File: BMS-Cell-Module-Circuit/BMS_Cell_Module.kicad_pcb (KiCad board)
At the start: 2 copper layers, 45.7 x 65.8 mm, 35 parts, among them J1 Conn_01x02_Female, J2 Conn_01x04_Female, J3 Conn_01x04_Female, M1 SI2312BDS-T1-E3, U2 ADUM1250ARZ, U3 ATTINY85V-10SU 8S2 EIAJ SOIC

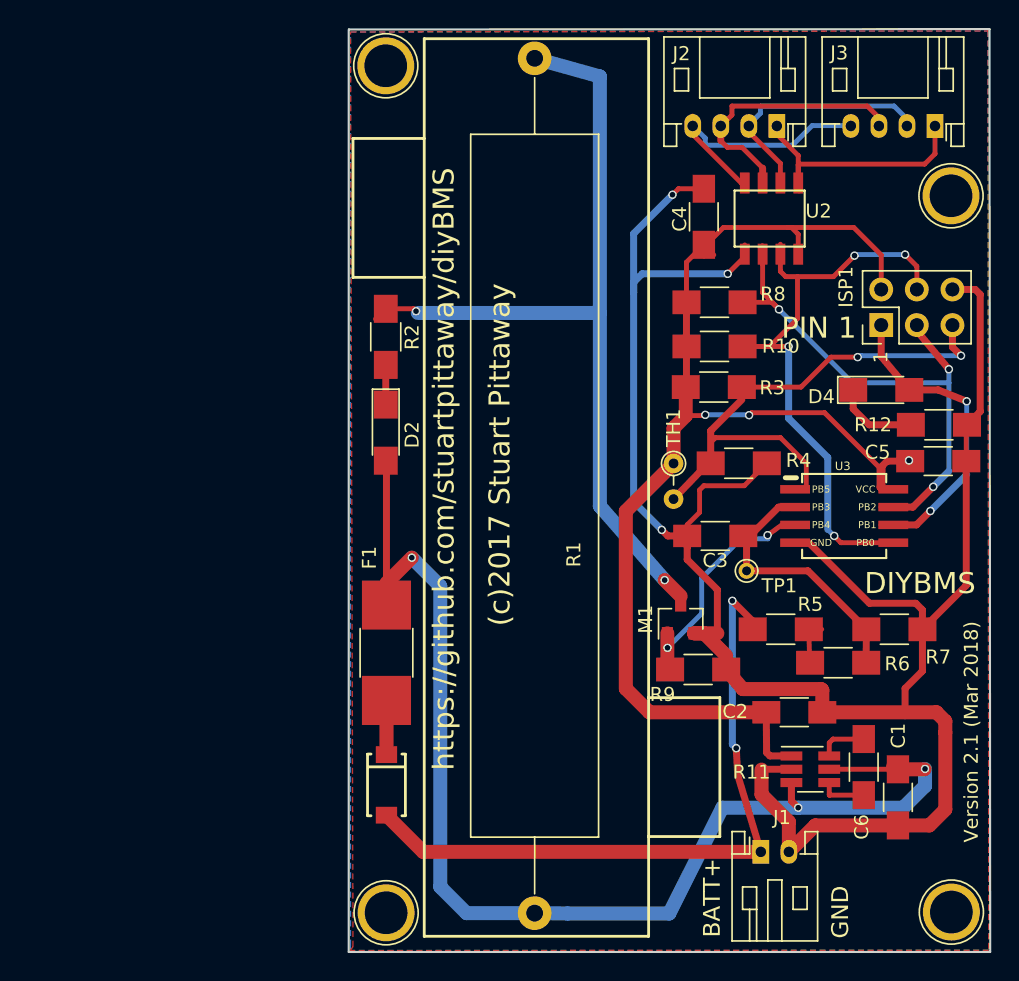
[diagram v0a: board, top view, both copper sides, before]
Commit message: First check in
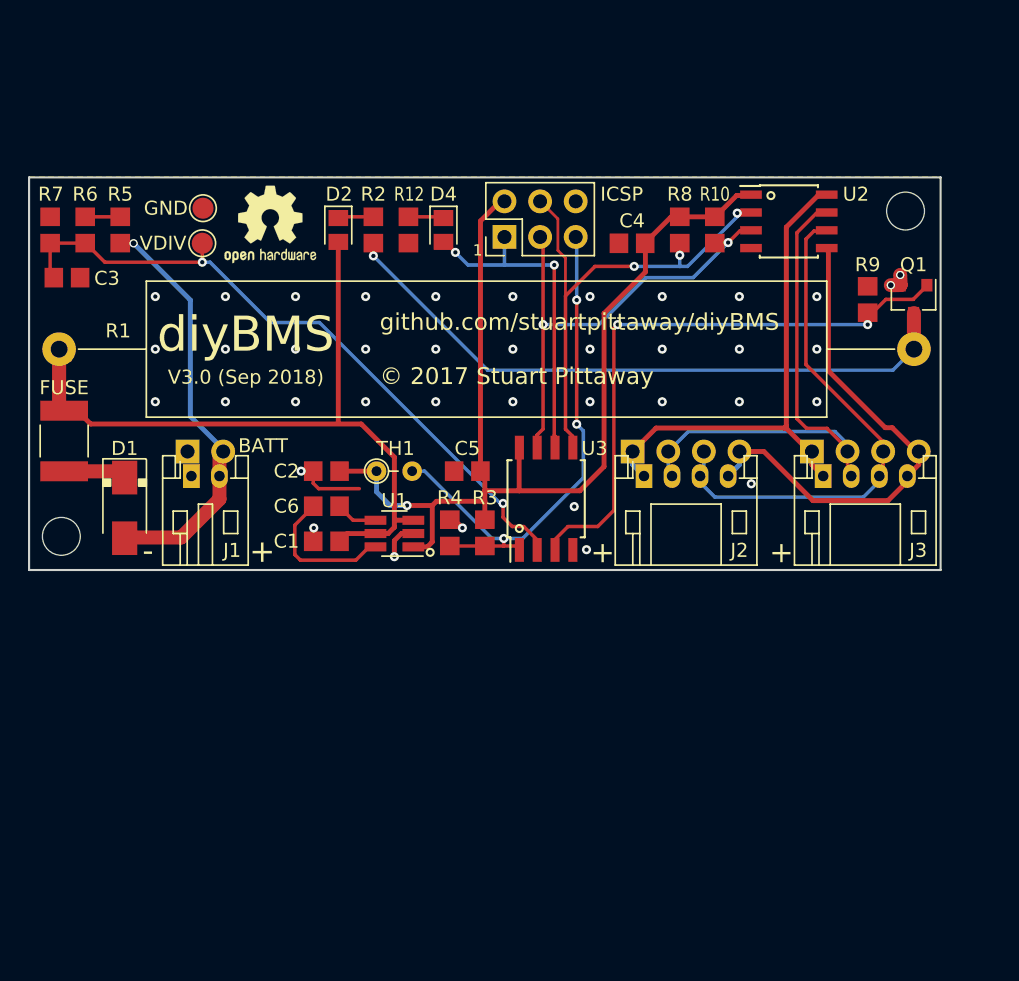
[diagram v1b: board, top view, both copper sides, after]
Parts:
- removed the J3 at (173.1, 67.3)
- removed M1: SI2312BDS-T1-E3, TO_SOT_Packages_SMD:SOT-23
- removed R11: REG710NA-3.3, TO_SOT_Packages_SMD:SOT-23-6_Handsoldering
- removed the REF** at (174.3, 123.4)
- removed the REF** at (134.0, 123.4)
- removed the REF** at (133.9, 63.0)
- added J2: Conn_01x04_Female, Connectors_JST:JST_PH_S4B-PH-K_04x2.00mm_Angled, F.Cu at (152.3, 92.3)
- added Q1: SI2312BDS-T1-E3, Package_TO_SOT_SMD:SOT-23, F.Cu at (171.6, 79.7)
- added REF**: PinHeader_1x04_P2.54mm_NoSilk, ATTINY:PinHeader_1x04_P2.54mm_NoSilk, F.Cu at (164.3, 90.5)
- added REF**: 2.7mm M2.5, MountingHole:MountingHole_2.7mm_M2.5, F.Cu at (110.8, 96.6)
- added REF**: OSHW-Logo2_7.3x6mm_SilkScreen, Symbol:OSHW-Logo2_7.3x6mm_SilkScreen, F.Cu at (125.7, 74.3)
- added REF**: PinHeader_1x04_P2.54mm_NoSilk, ATTINY:PinHeader_1x04_P2.54mm_NoSilk, F.Cu at (151.5, 90.5)
- added REF**: PinHeader_1x02_P2.54mm_NoSilk, ATTINY:PinHeader_1x02_P2.54mm_NoSilk, F.Cu at (119.8, 90.5)
- added TP2: TPGND, TestPoint:TestPoint_Pad_D1.5mm, F.Cu at (120.9, 73.2)
- added U1: REG710NA-3.3, TO_SOT_Packages_SMD:SOT-23-6_Handsoldering, F.Cu at (134.6, 96.4)
- C1, C2: value 2.2uF Ceramic X7R -> 2.2uF; footprint Capacitors_SMD:C_1206_HandSoldering -> Capacitor_SMD:C_0805_2012Metric_Pad1.33x1.40mm_HandSolder
- C3, C4, C5: footprint Capacitors_SMD:C_1206_HandSoldering -> Capacitor_SMD:C_0805_2012Metric_Pad1.33x1.40mm_HandSolder
- C6: value 0.22uF Ceramic X7R -> 0.22uF; footprint Capacitors_SMD:C_1206_HandSoldering -> Capacitor_SMD:C_0805_2012Metric_Pad1.33x1.40mm_HandSolder
- D1: value SE30AFG-M3/6A -> SS34 Schottky 40V/3A
- D2, D4: footprint LEDs:LED_1206_HandSoldering -> LED_SMD:LED_0805_2012Metric_Pad1.15x1.40mm_HandSolder
- F1: value MC36228 1.5A 8V -> FUSE; footprint Resistors_SMD:R_1812_HandSoldering -> Resistor_SMD:R_1812_4532Metric_Pad1.42x3.40mm_HandSolder
- R1: value HS50 3R3 J 50W Axial Wire Wound -> 2R/10W; footprint Resistors_THT:R_Axial_Power_L50.0mm_W9.0mm_P60.96mm -> ATTINY:R_Axial_Power_L48.0mm_W9.5mm_P60.96mm
- R10, R12, R4, R5, R6, R7, R8, R9: footprint Resistors_SMD:R_1206_HandSoldering -> Resistor_SMD:R_0805_2012Metric_Pad1.33x1.40mm_HandSolder
- R2: value 47R -> 2K; footprint Resistors_SMD:R_1206_HandSoldering -> Resistor_SMD:R_0805_2012Metric_Pad1.33x1.40mm_HandSolder
- R3: value 20K -> 68K; footprint Resistors_SMD:R_1206_HandSoldering -> Resistor_SMD:R_0805_2012Metric_Pad1.33x1.40mm_HandSolder
- REF**: value 1pin -> 2.7mm M2.5; footprint Connectors:1pin -> MountingHole:MountingHole_2.7mm_M2.5
- TP1: footprint Connectors:PINTST -> TestPoint:TestPoint_Pad_D1.5mm
- U2: footprint adum1250:ADUM1250 -> Package_SO:SOIC-8_3.9x4.9mm_P1.27mm
- U3: footprint ATTINY:ATTINY85V -> Package_SO:SOIJ-8_5.3x5.3mm_P1.27mm
- moved R7 66.6 mm to (110.0, 74.8), turned to 90 degrees
- moved R6 61.9 mm to (112.5, 74.8), turned to 270 degrees
- moved R5 55.0 mm to (115.0, 74.8), turned to 90 degrees
- moved C3 49.8 mm to (111.2, 78.2), turned to 0 degrees
- moved J1 48.7 mm to (120.1, 92.3)
- moved TP1 45.3 mm to (120.8, 75.7), turned to 180 degrees
- moved C1 44.7 mm to (129.7, 97.0), turned to 180 degrees
- moved C6 42.6 mm to (129.7, 94.5), turned to 0 degrees
- moved R12 40.3 mm to (135.6, 74.8), turned to 270 degrees
- moved C2 37.5 mm to (129.7, 92.0), turned to 180 degrees
- moved R1 34.1 mm to (171.6, 83.2), turned to 180 degrees
- moved C5 33.6 mm to (139.8, 92.0), turned to 180 degrees
- moved D4 33.2 mm to (138.1, 74.8), turned to 270 degrees
- moved R9 29.0 mm to (168.3, 79.7), turned to 90 degrees
- moved ISP1 27.6 mm to (142.4, 75.2)
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- renumbered J2 to J3
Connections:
- J1 pad 1: BATT+RAW -> GND
- J1 pad 2: GND -> BATT+RAW
- R10 pad 1: /SDA -> /SCK
- R8 pad 1: 3V3 -> /SDA
- R8 pad 2: /SCK -> 3V3
- U2 pad 1: Net-(J2-Pad1) -> 3V3
- U2 pad 2: Net-(J2-Pad2) -> /SDA
- U2 pad 3: Net-(J2-Pad3) -> /SCK
- U2 pad 4: Net-(J2-Pad4) -> GND
- U2 pad 5: GND -> Net-(J2-Pad4)
- U2 pad 6: /SCK -> Net-(J2-Pad3)
- U2 pad 7: /SDA -> Net-(J2-Pad2)
- U2 pad 8: 3V3 -> Net-(J2-Pad1)
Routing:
- net GND: track 164.5 -> 10.9 mm, vias 3 -> 39
- net Net-(C1-Pad1): track 93.3 -> 54.2 mm, vias 3 -> 0
- net Net-(C3-Pad1): track 21.1 -> 48.9 mm, vias 0 -> 2
- net /PB4BYPASS: track 17.6 -> 43.1 mm
- net Net-(J2-Pad2): track 18.9 -> 38.7 mm
- net BATT+RAW: track 49.6 -> 30.3 mm, vias 2 -> 1
- net Net-(J2-Pad3): track 19.5 -> 37.9 mm
- net Net-(J2-Pad1): track 18.7 -> 36.6 mm
- net 3V3: track 95.1 -> 79.2 mm, vias 3 -> 1
- net Net-(Q1-Pad3): track 61.6 -> 46.0 mm, vias 2 -> 1
- net Net-(J2-Pad4): track 20.7 -> 36.2 mm
- net /SDA: track 46.1 -> 36.8 mm, vias 4 -> 3
- net Net-(C6-Pad1): track 3.50 -> 10.3 mm
- net /SCK: track 41.2 -> 35.2 mm, vias 3 -> 2
- net Net-(D4-Pad1): track 6.63 -> 2.54 mm
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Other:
- board size 45.7 x 65.8 mm -> 65 x 28 mm
- net class Default: trace_width 0.35 -> 0.25; via_dia 0.6 -> 0.65; via_drill 0.4 -> 0.3
- net class Power added: clearance 0.3, trace_width 1, via_dia 2, via_drill 0.8
- net class PowerAT added: clearance 0.3, trace_width 0.35, via_dia 0.65, via_drill 0.3
- rule trace_min: 0.35 -> 0.25
- board text added: "+"
- board text added: "-"
- board text added: "1.8→4.35V/2A"
- board text added: "ATTINY85 PROGRAM"
- board text added: "BATT"
- board text added: "FUSE"
- board text added: "I2C IN"
- board text added: "I2C OUT"
- board text added: "M2.5"
- board text added: "SCL"
- board text added: "SDA"
- board text added: "TH1"
- board text added: "V3.0 (Sep 2018)"
- board text added: "diyBMS"
- board text added: "github.com/stuartpittaway/diyBMS Redesigned PCB by Nick Smith © 2017 Stuart Pittaway"
- board text added: "github.com/stuartpittaway/diyBMS © 2017 Stuart Pittaway"
- board text removed: "(c)2017 Stuart Pittaway"
- board text removed: "(c)2017 Stuart Pittaway #MadeInTheBlackCountry"
- board text removed: "BATT+"
- board text removed: "DIYBMS"
- board text removed: "GND"
- board text removed: "PIN 1"
- board text removed: "Version 2.1 (Mar 2018)"
- board text removed: "https://github.com/stuartpittaway/diyBMS"
